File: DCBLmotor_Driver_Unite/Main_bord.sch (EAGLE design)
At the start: 72 parts, among them CN1 DF11-16DP-2DSA, CN2 DF11-16DP-2DSA, CN3 DF11-4DP-2DSR, CN4 HIF3FC-10PA-2.54DSA(71), CN5 HIF3FC-10PA-2.54DSA(71), CN6 0430450612, CN7 0430450612, CN8 BM11B-SRSS-TB, IC1 TMPM370FYFG, IC2 MCP2561FD-E/MF, IC3 AM26C32CD, IC4 AM26C32CD, IC5 LTC2862A, SW1 CVS-02TB, SW2 EVQ-PE104K

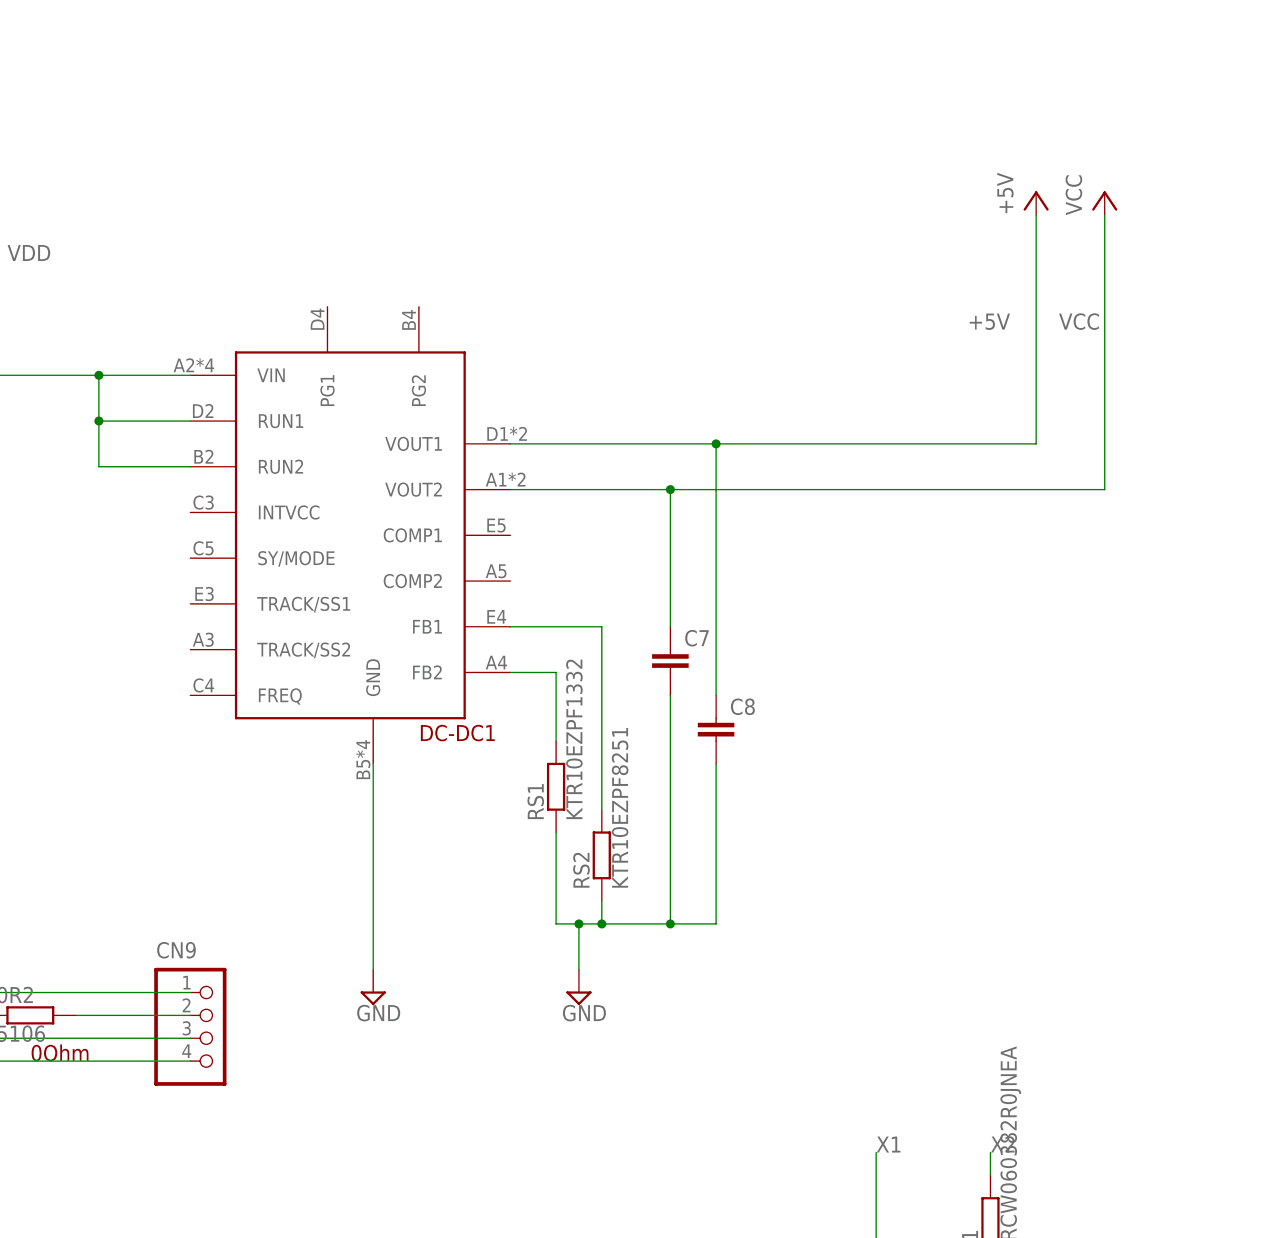
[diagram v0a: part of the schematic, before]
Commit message: TEMP Reples parts
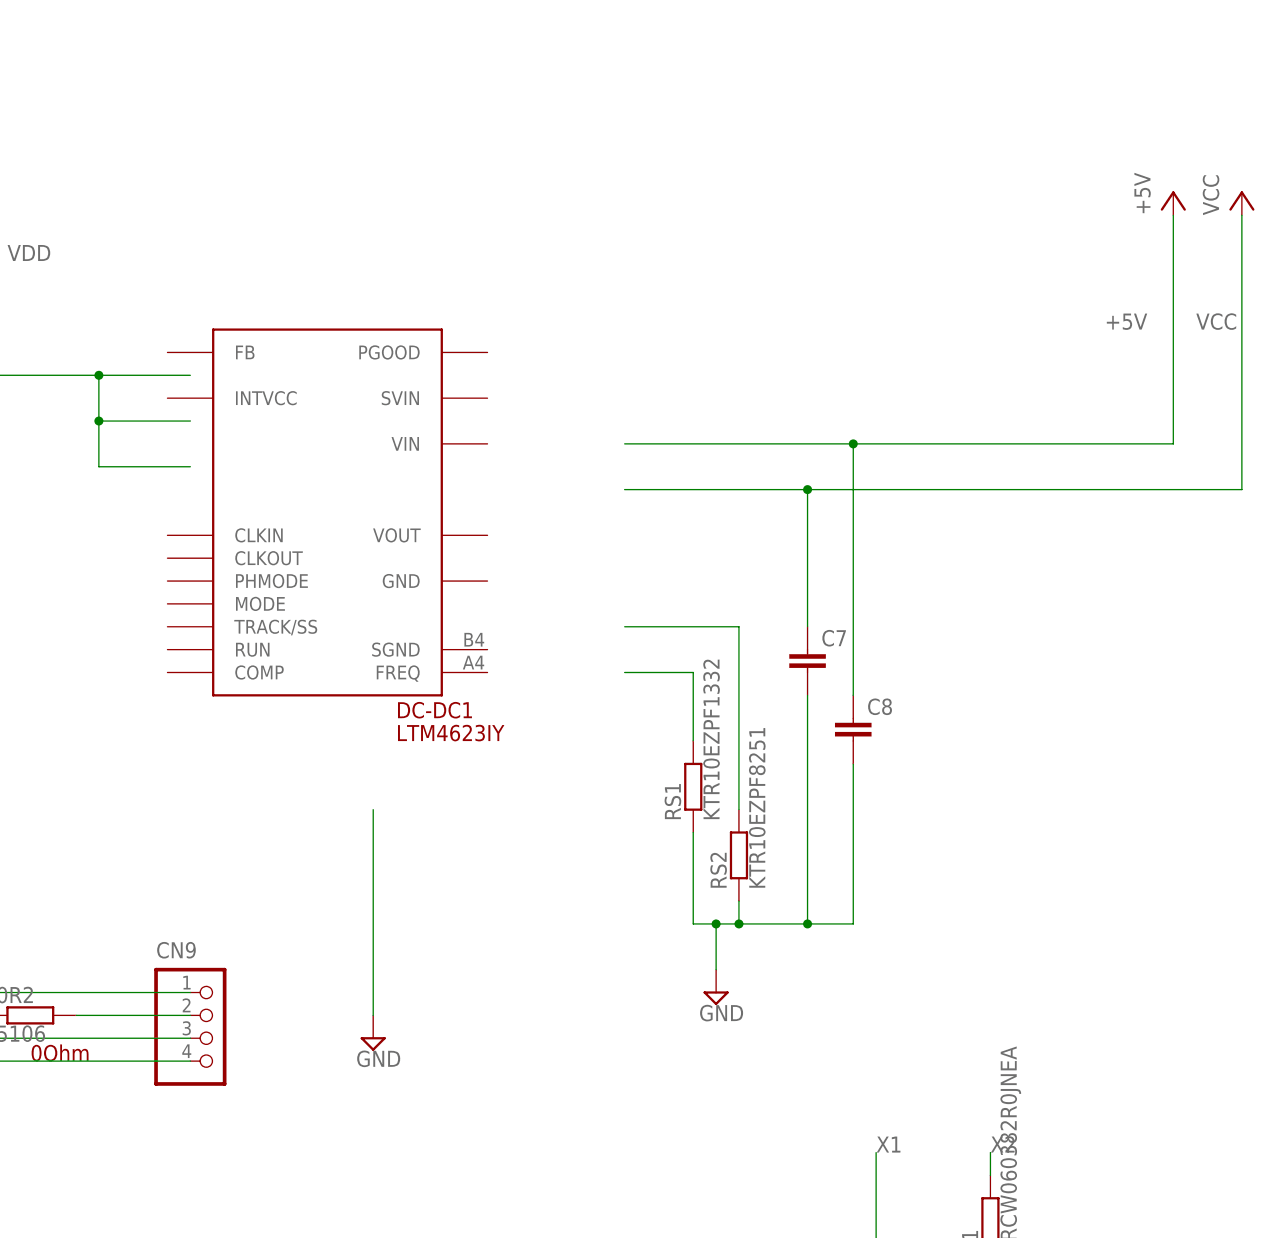
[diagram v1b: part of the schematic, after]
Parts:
- DC-DC1: value LTM4622 -> LTM4623IY; device LT:LTM4622 -> LT:LTM4623IY
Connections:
- net +5V: no longer DC-DC1.VOUT1
- net GND: no longer DC-DC1.GND
- net N$10: no longer DC-DC1.FB1
- net N$7: no longer DC-DC1.FB2
- net VCC: no longer DC-DC1.VOUT2
- net VDD: no longer DC-DC1.RUN1, DC-DC1.RUN2, DC-DC1.VIN
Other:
- moved on the sheet: C7, C8, RS1, RS2
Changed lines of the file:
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@@
 <part name="SUPPLY3" library="supply2" library_urn="urn:adsk.eagle:library:372" deviceset="GND" device=""/>
 <part name="SUPPLY5" library="supply2" library_urn="urn:adsk.eagle:library:372" deviceset="GND" device=""/>
-<part name="DC-DC1" library="LT" deviceset="LTM4622" device=""/>
 <part name="RS1" library="ROHM" deviceset="KTR10EZPF1332" device=""/>
 <part name="RS2" library="ROHM" deviceset="KTR10EZPF8251" device=""/>
@@
 <part name="CN10" library="jst-xh" deviceset="B2B-XH-A" device=""/>
 <part name="C5" library="KEMET" deviceset="T356L107K016AT" device=""/>
+<part name="DC-DC1" library="LT" deviceset="LTM4623IY" device=""/>
 </parts>
 <sheets>
@@
 <instance part="SUPPLY1" gate="GND" x="40.64" y="142.24"/>
 <instance part="SUPPLY2" gate="GND" x="231.14" y="20.32"/>
-<instance part="SUPPLY3" gate="GND" x="393.7" y="-17.78"/>
+<instance part="SUPPLY3" gate="GND" x="393.7" y="-22.86"/>
 <instance part="SUPPLY5" gate="GND" x="78.74" y="-127"/>
-<instance part="DC-DC1" gate="G$1" x="378.46" y="50.8"/>
-<instance part="RS1" gate="G$1" x="414.02" y="5.08" rot="R90"/>
-<instance part="RS2" gate="G$1" x="419.1" y="-2.54" rot="R90"/>
-<instance part="SUPPLY8" gate="GND" x="416.56" y="-17.78"/>
-<instance part="C7" gate="G$1" x="426.72" y="20.32"/>
-<instance part="C8" gate="G$1" x="431.8" y="12.7"/>
+<instance part="RS1" gate="G$1" x="429.26" y="5.08" rot="R90"/>
+<instance part="RS2" gate="G$1" x="434.34" y="-2.54" rot="R90"/>
+<instance part="SUPPLY8" gate="GND" x="431.8" y="-17.78"/>
+<instance part="C7" gate="G$1" x="441.96" y="20.32"/>
+<instance part="C8" gate="G$1" x="447.04" y="12.7"/>
 <instance part="CR1" gate="G$1" x="246.38" y="38.1"/>
 <instance part="CR3" gate="G$1" x="231.14" y="30.48"/>
@@
 <instance part="SUPPLY9" gate="GND" x="246.38" y="20.32"/>
 <instance part="SUPPLY10" gate="GND" x="-127" y="7.62"/>
-<instance part="P+6" gate="VCC" x="474.98" y="71.12"/>
-<instance part="P+7" gate="VCC" x="467.36" y="71.12"/>
+<instance part="P+6" gate="VCC" x="490.22" y="71.12"/>
+<instance part="P+7" gate="VCC" x="482.6" y="71.12"/>
 <instance part="SUPPLY4" gate="G$1" x="347.98" y="71.12"/>
 <instance part="SUPPLY11" gate="GND" x="-35.56" y="96.52"/>
@@
 <instance part="CN10" gate="G$1" x="467.36" y="220.98"/>
 <instance part="C5" gate="G$1" x="439.42" y="220.98"/>
+<instance part="DC-DC1" gate="G$1" x="388.62" y="35.56"/>
 </instances>
 <busses>
@@
 <net name="GND" class="0">
 <segment>
-<pinref part="DC-DC1" gate="G$1" pin="GND"/>
 <pinref part="SUPPLY3" gate="GND" pin="GND"/>
-<wire x1="393.7" y1="7.62" x2="393.7" y2="-15.24" width="0.1524" layer="91"/>
+<wire x1="393.7" y1="2.54" x2="393.7" y2="-20.32" width="0.1524" layer="91"/>
 </segment>
 <segment>
 <pinref part="RS1" gate="G$1" pin="2"/>
-<wire x1="414.02" y1="0" x2="414.02" y2="-10.16" width="0.1524" layer="91"/>
+<wire x1="429.26" y1="0" x2="429.26" y2="-10.16" width="0.1524" layer="91"/>
 <pinref part="RS2" gate="G$1" pin="2"/>
-<wire x1="419.1" y1="-7.62" x2="419.1" y2="-10.16" width="0.1524" layer="91"/>
-<wire x1="419.1" y1="-10.16" x2="416.56" y2="-10.16" width="0.1524" layer="91"/>
+<wire x1="434.34" y1="-7.62" x2="434.34" y2="-10.16" width="0.1524" layer="91"/>
+<wire x1="434.34" y1="-10.16" x2="431.8" y2="-10.16" width="0.1524" layer="91"/>
 <pinref part="SUPPLY8" gate="GND" pin="GND"/>
-<wire x1="416.56" y1="-10.16" x2="414.02" y2="-10.16" width="0.1524" layer="91"/>
-<wire x1="416.56" y1="-10.16" x2="416.56" y2="-15.24" width="0.1524" layer="91"/>
-<junction x="416.56" y="-10.16"/>
+<wire x1="431.8" y1="-10.16" x2="429.26" y2="-10.16" width="0.1524" layer="91"/>
+<wire x1="431.8" y1="-10.16" x2="431.8" y2="-15.24" width="0.1524" layer="91"/>
+<junction x="431.8" y="-10.16"/>
 <pinref part="C8" gate="G$1" pin="2"/>
-<wire x1="419.1" y1="-10.16" x2="426.72" y2="-10.16" width="0.1524" layer="91"/>
-<wire x1="426.72" y1="-10.16" x2="431.8" y2="-10.16" width="0.1524" layer="91"/>
-<wire x1="431.8" y1="-10.16" x2="431.8" y2="7.62" width="0.1524" layer="91"/>
-<junction x="419.1" y="-10.16"/>
+<wire x1="434.34" y1="-10.16" x2="441.96" y2="-10.16" width="0.1524" layer="91"/>
+<wire x1="441.96" y1="-10.16" x2="447.04" y2="-10.16" width="0.1524" layer="91"/>
+<wire x1="447.04" y1="-10.16" x2="447.04" y2="7.62" width="0.1524" layer="91"/>
+<junction x="434.34" y="-10.16"/>
 <pinref part="C7" gate="G$1" pin="2"/>
-<wire x1="426.72" y1="15.24" x2="426.72" y2="-10.16" width="0.1524" layer="91"/>
-<junction x="426.72" y="-10.16"/>
+<wire x1="441.96" y1="15.24" x2="441.96" y2="-10.16" width="0.1524" layer="91"/>
+<junction x="441.96" y="-10.16"/>
 </segment>
 <segment>
@@
 <net name="N$7" class="0">
 <segment>
-<pinref part="DC-DC1" gate="G$1" pin="FB2"/>
 <pinref part="RS1" gate="G$1" pin="1"/>
-<wire x1="408.94" y1="17.78" x2="414.02" y2="17.78" width="0.1524" layer="91"/>
-<wire x1="414.02" y1="17.78" x2="414.02" y2="10.16" width="0.1524" layer="91"/>
+<wire x1="421.64" y1="17.78" x2="429.26" y2="17.78" width="0.1524" layer="91"/>
+<wire x1="429.26" y1="17.78" x2="429.26" y2="10.16" width="0.1524" layer="91"/>
 </segment>
 </net>
 <net name="N$10" class="0">
 <segment>
-<pinref part="DC-DC1" gate="G$1" pin="FB1"/>
 <pinref part="RS2" gate="G$1" pin="1"/>
-<wire x1="408.94" y1="22.86" x2="419.1" y2="22.86" width="0.1524" layer="91"/>
-<wire x1="419.1" y1="22.86" x2="419.1" y2="2.54" width="0.1524" layer="91"/>
+<wire x1="421.64" y1="22.86" x2="434.34" y2="22.86" width="0.1524" layer="91"/>
+<wire x1="434.34" y1="22.86" x2="434.34" y2="2.54" width="0.1524" layer="91"/>
 </segment>
 </net>
@@
 <segment>
 <pinref part="P+6" gate="VCC" pin="VCC"/>
-<wire x1="474.98" y1="68.58" x2="474.98" y2="38.1" width="0.1524" layer="91"/>
-<label x="469.9" y="55.88" size="1.778" layer="95"/>
-<wire x1="426.72" y1="38.1" x2="474.98" y2="38.1" width="0.1524" layer="91"/>
+<wire x1="490.22" y1="68.58" x2="490.22" y2="38.1" width="0.1524" layer="91"/>
+<label x="485.14" y="55.88" size="1.778" layer="95"/>
+<wire x1="441.96" y1="38.1" x2="490.22" y2="38.1" width="0.1524" layer="91"/>
 <pinref part="C7" gate="G$1" pin="1"/>
-<pinref part="DC-DC1" gate="G$1" pin="VOUT2"/>
-<wire x1="426.72" y1="22.86" x2="426.72" y2="38.1" width="0.1524" layer="91"/>
-<wire x1="426.72" y1="38.1" x2="408.94" y2="38.1" width="0.1524" layer="91"/>
-<junction x="426.72" y="38.1"/>
+<wire x1="441.96" y1="22.86" x2="441.96" y2="38.1" width="0.1524" layer="91"/>
+<wire x1="441.96" y1="38.1" x2="421.64" y2="38.1" width="0.1524" layer="91"/>
+<junction x="441.96" y="38.1"/>
 </segment>
 <segment>
@@
 <segment>
 <pinref part="P+7" gate="VCC" pin="VCC"/>
-<wire x1="467.36" y1="68.58" x2="467.36" y2="43.18" width="0.1524" layer="91"/>
-<label x="459.74" y="55.88" size="1.778" layer="95"/>
-<pinref part="DC-DC1" gate="G$1" pin="VOUT1"/>
+<wire x1="482.6" y1="68.58" x2="482.6" y2="43.18" width="0.1524" layer="91"/>
+<label x="474.98" y="55.88" size="1.778" layer="95"/>
 <pinref part="C8" gate="G$1" pin="1"/>
-<wire x1="408.94" y1="43.18" x2="431.8" y2="43.18" width="0.1524" layer="91"/>
-<wire x1="431.8" y1="43.18" x2="431.8" y2="15.24" width="0.1524" layer="91"/>
-<junction x="431.8" y="43.18"/>
-<wire x1="431.8" y1="43.18" x2="467.36" y2="43.18" width="0.1524" layer="91"/>
+<wire x1="421.64" y1="43.18" x2="447.04" y2="43.18" width="0.1524" layer="91"/>
+<wire x1="447.04" y1="43.18" x2="447.04" y2="15.24" width="0.1524" layer="91"/>
+<junction x="447.04" y="43.18"/>
+<wire x1="447.04" y1="43.18" x2="482.6" y2="43.18" width="0.1524" layer="91"/>
 </segment>
 <segment>
@@
 <wire x1="347.98" y1="68.58" x2="347.98" y2="50.8" width="0.1524" layer="91"/>
 <label x="353.06" y="63.5" size="1.778" layer="95"/>
-<pinref part="DC-DC1" gate="G$1" pin="VIN"/>
 <wire x1="373.38" y1="50.8" x2="363.22" y2="50.8" width="0.1524" layer="91"/>
-<pinref part="DC-DC1" gate="G$1" pin="RUN2"/>
 <wire x1="363.22" y1="50.8" x2="347.98" y2="50.8" width="0.1524" layer="91"/>
 <wire x1="373.38" y1="40.64" x2="363.22" y2="40.64" width="0.1524" layer="91"/>
 <wire x1="363.22" y1="40.64" x2="363.22" y2="45.72" width="0.1524" layer="91"/>
 <junction x="363.22" y="50.8"/>
-<pinref part="DC-DC1" gate="G$1" pin="RUN1"/>
 <wire x1="363.22" y1="45.72" x2="363.22" y2="50.8" width="0.1524" layer="91"/>
 <wire x1="373.38" y1="45.72" x2="363.22" y2="45.72" width="0.1524" layer="91"/>
